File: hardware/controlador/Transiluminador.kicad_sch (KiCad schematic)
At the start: 84 parts, among them J1 Conn_01x01_Pin, J10 USB_B_Micro, J11 HDR-2x1, J12 Conn_01x02, J3 HDR-2x1, J7 HDR-3x1, J9 HDR-3x1, Q1 Q_PMOS_GSD, Q2 NPN, Q4 Q_Dual_NPN_NPN_BRT_E1B1C2E2B2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, SW2 SW_DIP_x02, SW3 SW_DIP_x02, U1 ${SIM.PARAMS}, U10 ESP32-WROOM-32D, U11 RV-8803, U4 MT3608, U6 AP2112K-3.3, U7 AP2112K-3.3, U8 AP2112K-3.3, U9 CH340C

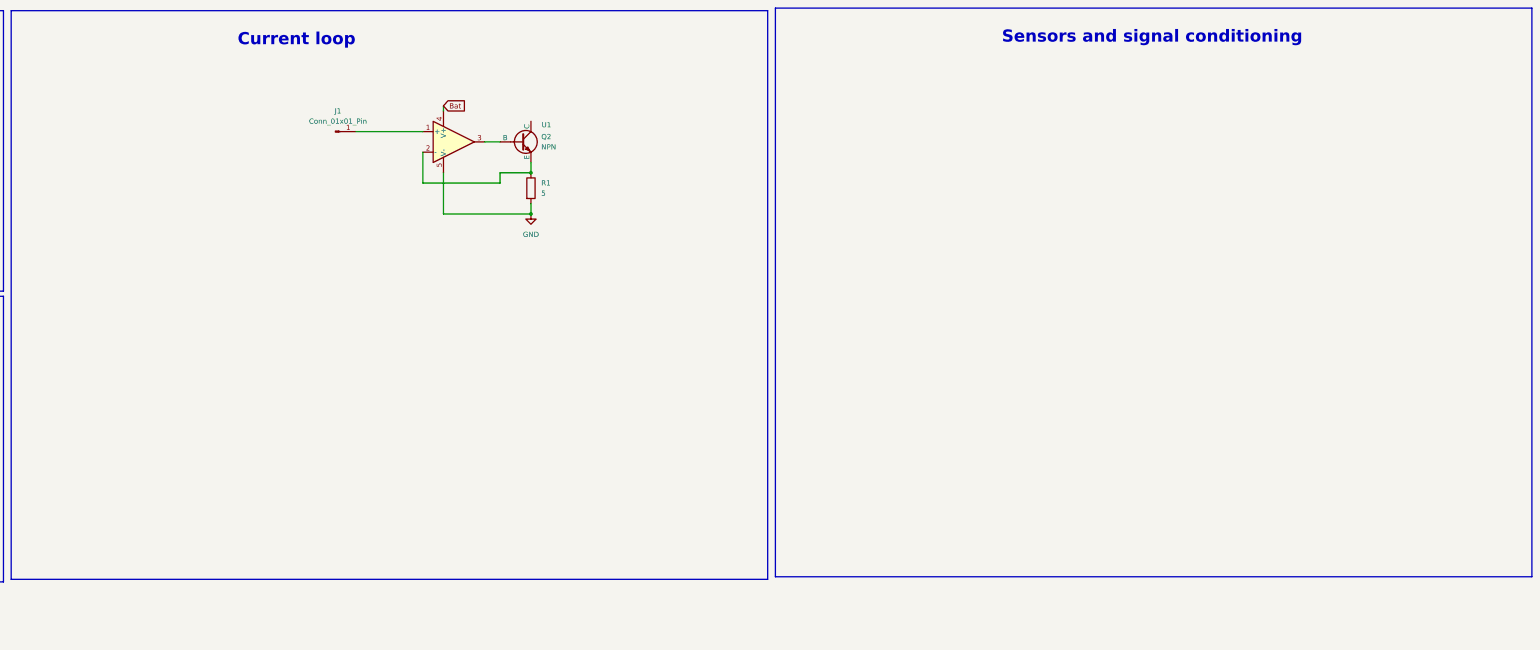
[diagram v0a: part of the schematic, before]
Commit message: actualización
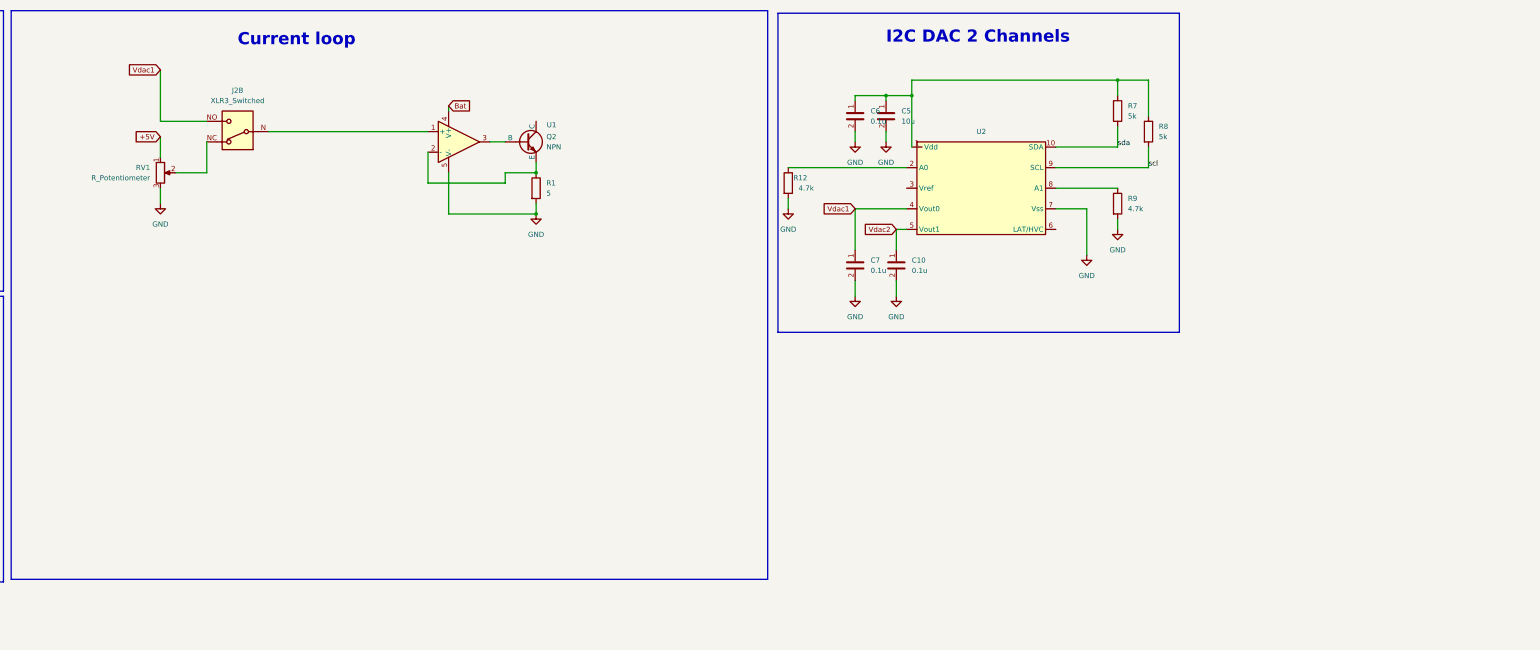
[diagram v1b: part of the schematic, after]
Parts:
- removed J1: Conn_01x01_Pin, Connector_PinHeader_1.00mm:PinHeader_1x01_P1.00mm_Horizontal, symbol Connector:Conn_01x01_Pin
- added C10, C6, C7: 0.1u, Capacitor_SMD:C_0603_1608Metric, symbol IoWLabs:C
- added C5: 10u, Capacitor_SMD:C_0603_1608Metric, symbol IoWLabs:C
- added J2: XLR3_Switched, symbol Connector_Audio:XLR3_Switched
- added R12, R9: 4.7k, symbol Device:R
- added R7, R8: 5k, symbol Device:R
- added RV1: R_Potentiometer, symbol Device:R_Potentiometer
- added U2: ~, Package_SO:MSOP-10_3x3mm_P0.5mm, symbol IoWLabs:MCP47CB
- C3: footprint (none) -> Capacitor_SMD:C_0603_1608Metric
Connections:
- net +5V: now also RV1.1
- net GND: now also C10.2, C5.2, C6.2, C7.2, R12.2, R9.2, RV1.3, U2.7 (Vss)
- net scl: now also R8.2, U2.9 (SCL)
- net sda: now also R7.2, U2.10 (SDA)
- net at U1.1 (+): now also J2.N
- new net: C5.1, C6.1, R7.1, R8.1, U2.1 (Vdd)
- new net: R12.1, U2.2 (A0)
- new net: R9.1, U2.8 (A1)
- new net: J2.NC, RV1.2
- new net Vdac1: C7.1, J2.NO, U2.4 (Vout0)
- new net Vdac2: C10.1, U2.5 (Vout1)
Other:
- note added: "I2C DAC 2 Channels"
- note removed: "Sensors and signal conditioning"
- moved on the sheet: Q2, R1, U1
